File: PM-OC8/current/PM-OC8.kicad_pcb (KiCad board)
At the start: 2 copper layers, 25.4 x 53.3 mm, 26 parts, among them J1 Conn_01x10_Pin, J2 Conn_01x10_Pin, U1 PC817, U2 PC817, U3 PC817, U4 PC817, U5 PC817, U6 PC817, U7 PC817, U8 PC817

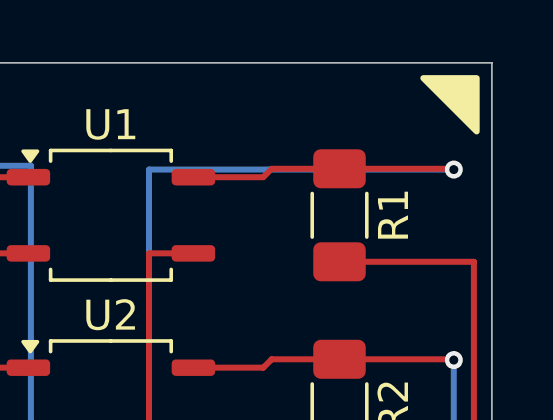
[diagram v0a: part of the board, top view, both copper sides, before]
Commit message: sync
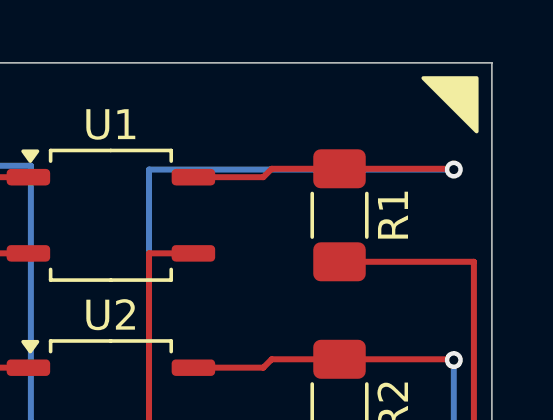
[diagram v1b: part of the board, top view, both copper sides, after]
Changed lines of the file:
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@@
 			(pdf_front_fp_property_popups yes)
 			(pdf_back_fp_property_popups yes)
-			(dxfpolygonmode yes)
+			(dxfpolygonmode no)
 			(dxfimperialunits yes)
 			(dxfusepcbnewfont yes)
@@
 			(sketchpadsonfab no)
 			(subtractmaskfromsilk no)
-			(outputformat 1)
+			(outputformat 4)
 			(mirror no)
 			(drillshape 0)
@@
 		)
 		(stroke
-			(width 0.2)
+			(width 0.127)
 			(type solid)
 		)
